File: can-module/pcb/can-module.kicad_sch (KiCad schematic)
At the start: 28 parts, among them IC1 PIC32CM1216JH01048-I_U5B, J1 Conn_01x08_Socket, J2 Conn_01x02_Socket, J3 Conn_01x04_Socket, U1 ATA6560-GBQW-N

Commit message: can-module: Update CAN/PWR header to also be 0.127mm, move some things around to allow for wider min power plane width
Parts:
- J3: footprint Conn01x04:01x04_1mm -> Connector_PinHeader_1.27mm:PinHeader_1x04_P1.27mm_Vertical
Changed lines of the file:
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@@
 			)
 		)
-		(property "Footprint" "Conn01x04:01x04_1mm"
+		(property "Footprint" "Connector_PinHeader_1.27mm:PinHeader_1x04_P1.27mm_Vertical"
 			(at 209.55 41.91 0)
 			(effects

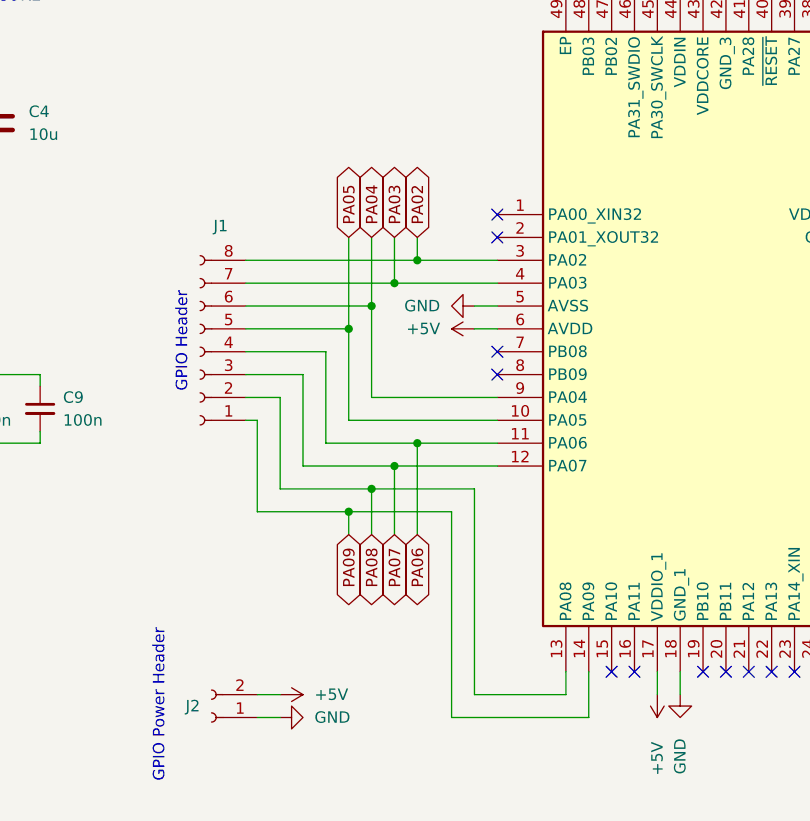
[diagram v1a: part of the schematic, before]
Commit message: can-module, pmod-adapter: Begin updating PMOD adapter and CAN module
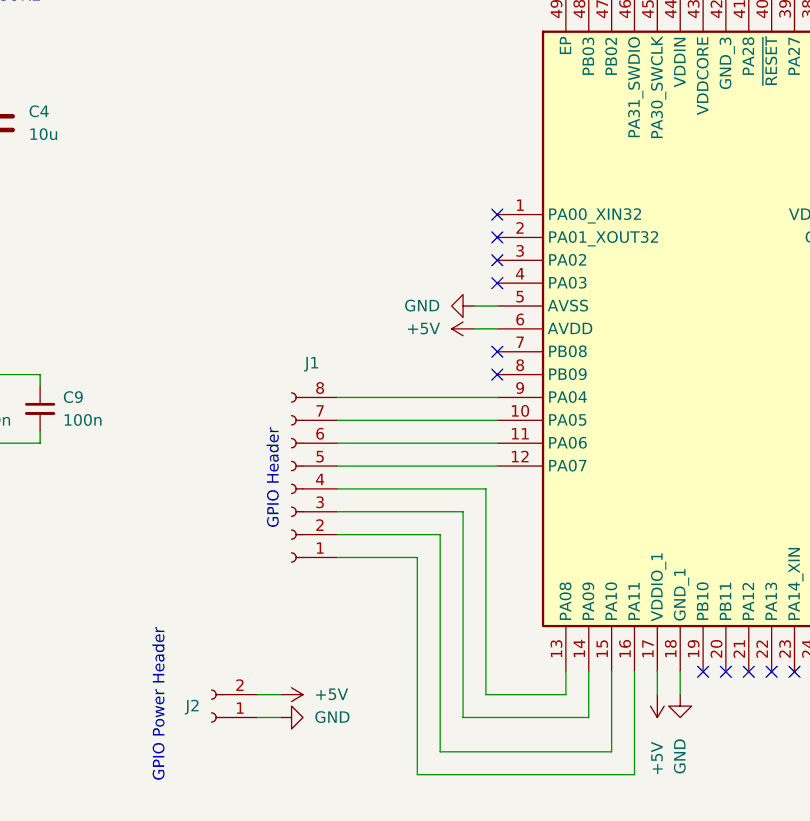
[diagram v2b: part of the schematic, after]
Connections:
- net at IC1.15 (PA10): now also J1.2 (Pin_2)
- net at IC1.16 (PA11): now also J1.1 (Pin_1)
- net PA02: no longer names the net of IC1.3 (PA02)
- net PA02: no longer J1.8 (Pin_8)
- net PA03: no longer names the net of J1.7 (Pin_7)
- net PA03: now also IC1.10 (PA05); no longer IC1.4 (PA03)
- net PA04: no longer names the net of J1.6 (Pin_6)
- net PA04: now also IC1.11 (PA06); no longer IC1.9 (PA04)
- net PA05: no longer names the net of J1.5 (Pin_5)
- net PA05: now also IC1.12 (PA07); no longer IC1.10 (PA05)
- net PA06: no longer names the net of J1.4 (Pin_4)
- net PA06: now also IC1.13 (PA08); no longer IC1.11 (PA06)
- net PA07: no longer names the net of J1.3 (Pin_3)
- net PA07: now also IC1.14 (PA09); no longer IC1.12 (PA07)
- removed net PA08: IC1.13 (PA08), J1.2 (Pin_2)
- removed net PA09: IC1.14 (PA09), J1.1 (Pin_1)
- new net: IC1.9 (PA04), J1.8 (Pin_8)
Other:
- moved on the sheet: J1
